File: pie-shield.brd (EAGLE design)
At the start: 35.5 x 56.2 mm, 15 parts, among them IC6 78L05, IC8 MAX487, X6 RJ45-8L-B

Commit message: before wiring to raspberry
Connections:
- net N$35 renamed SELECT
- net +5V: now also U$2.P1_2, U$2.P1_4, U$2.P5_1
- net GND: now also U$2.P1_14, U$2.P1_20, U$2.P1_6, U$2.P5_7, U$2.P5_8
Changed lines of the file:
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@@
 <contactref element="R22" pad="1"/>
 <contactref element="R19" pad="1"/>
-<wire x1="25.3475" y1="38.1" x2="33.92" y2="40.64" width="0" layer="19" extent="1-1"/>
-<wire x1="28.575" y1="34.8234" x2="25.3475" y2="38.1" width="0" layer="19" extent="1-1"/>
-<wire x1="29.845" y1="34.8234" x2="28.575" y2="34.8234" width="0" layer="19" extent="1-1"/>
+<contactref element="U$2" pad="P1_2"/>
+<contactref element="U$2" pad="P1_4"/>
+<contactref element="U$2" pad="P5_1"/>
+<wire x1="29.845" y1="34.8234" x2="33.92" y2="40.64" width="0" layer="19" extent="1-1"/>
+<wire x1="28.575" y1="34.8234" x2="29.845" y2="34.8234" width="0" layer="19" extent="1-1"/>
+<wire x1="25.3475" y1="38.1" x2="28.575" y2="34.8234" width="0" layer="19" extent="1-1"/>
 <wire x1="17.7275" y1="38.1" x2="25.3475" y2="38.1" width="0" layer="19" extent="1-1"/>
+<wire x1="7.62" y1="48.26" x2="17.7275" y2="38.1" width="0" layer="19" extent="1-1"/>
+<wire x1="5.08" y1="53.34" x2="7.62" y2="48.26" width="0" layer="19" extent="1-1"/>
+<wire x1="2.54" y1="53.34" x2="5.08" y2="53.34" width="0" layer="19" extent="1-1"/>
 </signal>
-<signal name="N$35">
+<signal name="SELECT">
 <contactref element="OK3" pad="3"/>
 </signal>
@@
 <contactref element="OK2" pad="5"/>
 <contactref element="C24" pad="1"/>
+<contactref element="U$2" pad="P1_14"/>
+<contactref element="U$2" pad="P1_20"/>
+<contactref element="U$2" pad="P5_8"/>
+<contactref element="U$2" pad="P5_7"/>
+<contactref element="U$2" pad="P1_6"/>
+<wire x1="17.78" y1="53.34" x2="25.4" y2="53.34" width="0" layer="19" extent="1-1"/>
+<wire x1="15.24" y1="48.26" x2="17.78" y2="53.34" width="0" layer="19" extent="1-1"/>
+<wire x1="15.24" y1="45.72" x2="15.24" y2="48.26" width="0" layer="19" extent="1-1"/>
+<wire x1="7.62" y1="53.34" x2="15.24" y2="48.26" width="0" layer="19" extent="1-1"/>
+<wire x1="32.12" y1="40.64" x2="25.4" y2="53.34" width="0" layer="19" extent="1-1"/>
+<wire x1="32.385" y1="34.8234" x2="32.12" y2="40.64" width="0" layer="19" extent="1-1"/>
 </signal>
 </signals>

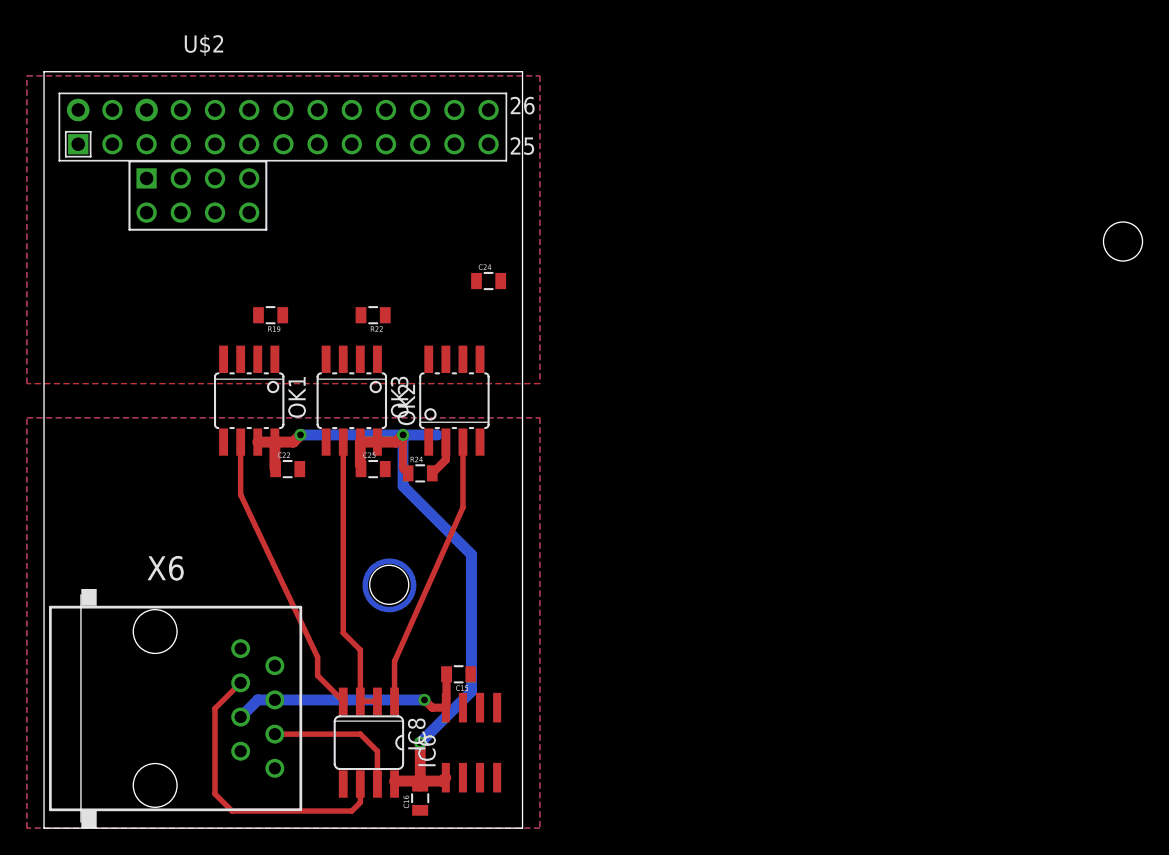
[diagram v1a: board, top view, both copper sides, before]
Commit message: wired
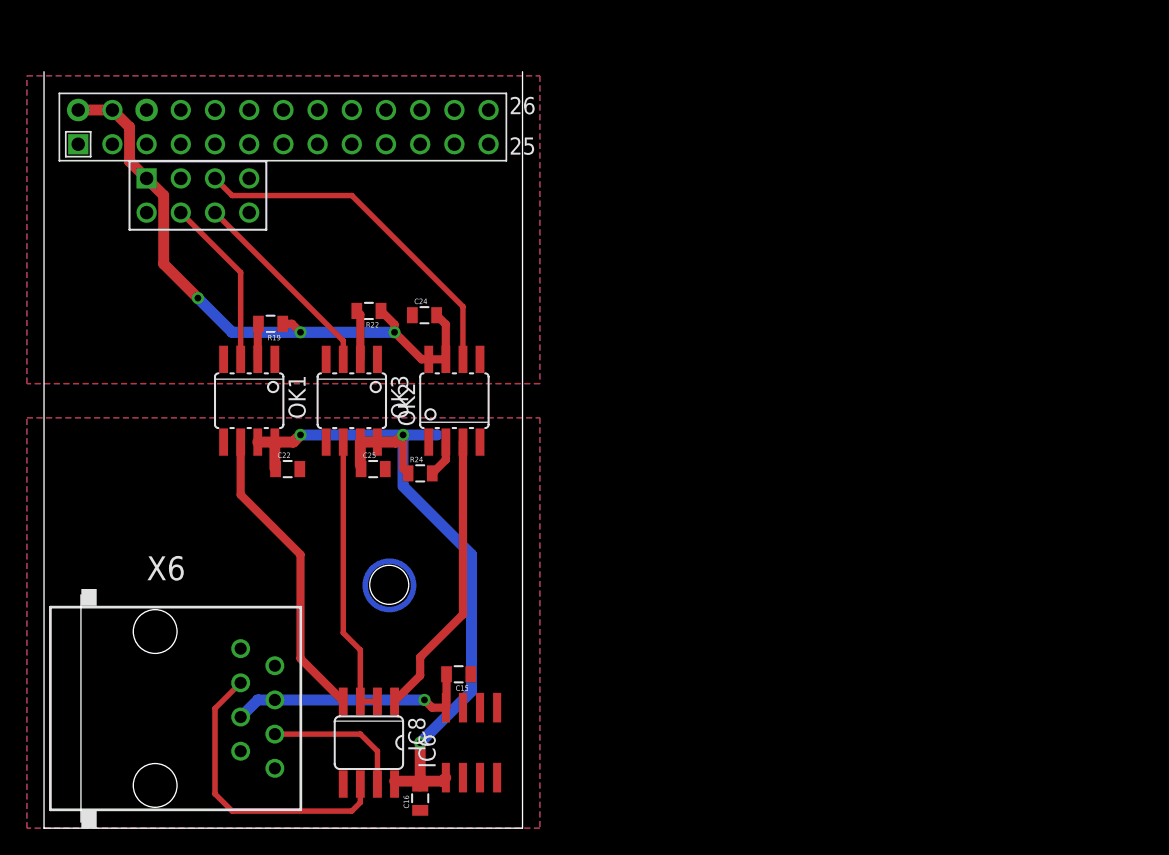
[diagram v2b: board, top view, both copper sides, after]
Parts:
- moved C24 5.40 mm to (28.3, 38.1)
- moved R19 0.63 mm to (16.8, 37.5)
- moved R22 0.45 mm to (24.1, 38.4)
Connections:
- net RXD_AL: now also U$2.P5_5
- net SELECT: now also U$2.P5_6
- net TXD_AL: now also U$2.P5_4
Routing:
- net +5V: track 0.00 -> 46.6 mm, vias 0 -> 3
- net RXD_AL: track 0.00 -> 26.3 mm
- net SELECT: track 0.00 -> 14.8 mm
- net TXD_AL: track 0.00 -> 12.7 mm
- net N$44: track 0.00 -> 3.70 mm
- net N$32: track 0.00 -> 2.66 mm
- net TXD1: track 21.3 -> 22.4 mm
- net RXD1: track 20.3 -> 21.4 mm
